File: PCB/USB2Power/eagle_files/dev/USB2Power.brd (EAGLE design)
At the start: 12.5 x 20 mm, 7 parts, among them SW1 PCM12SMTR

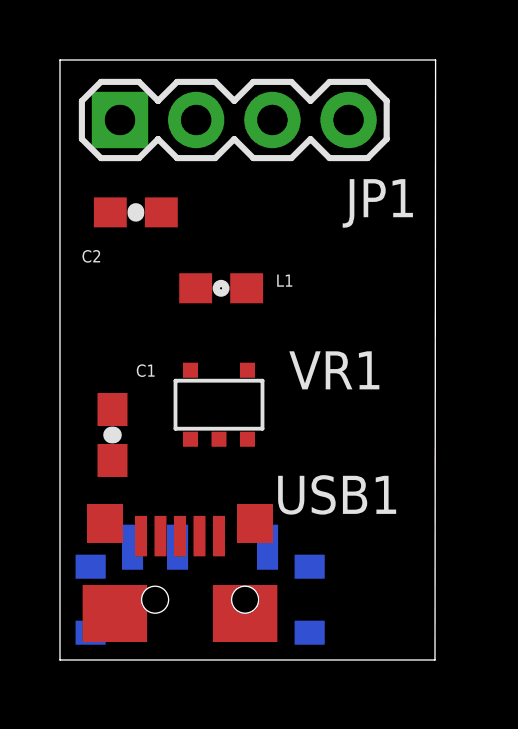
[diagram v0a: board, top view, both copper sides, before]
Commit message: USB2Power board components placed and ready for routing.
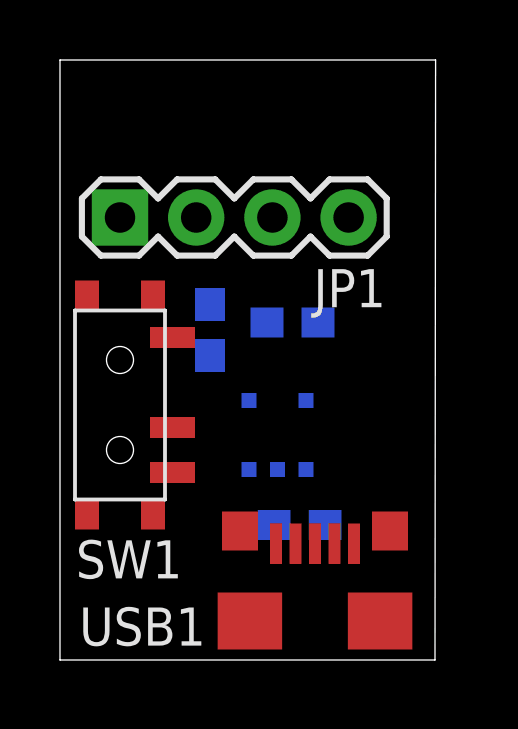
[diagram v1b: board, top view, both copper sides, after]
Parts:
- moved SW1 7.02 mm to (2.00, 8.50), flipped to the top, turned to 270 degrees
- moved C1 6.92 mm to (7.99, 4.50), flipped to the bottom, turned to 180 degrees
- moved C2 4.63 mm to (5.00, 11.0), flipped to the bottom, turned to 270 degrees
- moved USB1 4.51 mm to (8.50, 2.25)
- moved JP1 3.25 mm to (2.00, 14.8)
- moved L1 2.64 mm to (7.75, 11.2), flipped to the bottom
- moved VR1 2.20 mm to (7.25, 7.50), flipped to the bottom
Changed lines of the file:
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@@
 </autorouter>
 <elements>
-<element name="C1" library="SparkFun-Capacitors" package="0603-CAP" value="" x="1.75" y="7.5" smashed="yes" rot="R270">
-<attribute name="NAME" x="2.531" y="9.442" size="0.4064" layer="25" font="vector"/>
-<attribute name="VALUE" x="0.607" y="8.516" size="0.4064" layer="27" font="vector" rot="R270"/>
+<element name="C1" library="SparkFun-Capacitors" package="0603-CAP" value="" x="7.99" y="4.5" smashed="yes" rot="MR180">
+<attribute name="NAME" x="5.711" y="3.318" size="0.4064" layer="26" font="vector" rot="MR180"/>
+<attribute name="VALUE" x="6.974" y="5.643" size="0.4064" layer="28" font="vector" rot="MR180"/>
 </element>
-<element name="C2" library="SparkFun-Capacitors" package="0603-CAP" value="" x="2.53" y="14.92" smashed="yes">
-<attribute name="NAME" x="0.721" y="13.252" size="0.4064" layer="25" font="vector"/>
-<attribute name="VALUE" x="1.514" y="13.777" size="0.4064" layer="27" font="vector"/>
+<element name="C2" library="SparkFun-Capacitors" package="0603-CAP" value="" x="5" y="11" smashed="yes" rot="MR270">
+<attribute name="NAME" x="4.021" y="13.058" size="0.4064" layer="26" font="vector" rot="MR180"/>
+<attribute name="VALUE" x="6.143" y="12.016" size="0.4064" layer="28" font="vector" rot="MR270"/>
 </element>
-<element name="JP1" library="SparkFun-Connectors" package="1X04" value="" x="2" y="18" smashed="yes">
-<attribute name="NAME" x="9.5038" y="14.7588" size="1.27" layer="25" ratio="10"/>
-<attribute name="VALUE" x="0.73" y="14.825" size="1.27" layer="27"/>
+<element name="JP1" library="SparkFun-Connectors" package="1X04" value="" x="2" y="14.75" smashed="yes">
+<attribute name="NAME" x="8.4538" y="11.7588" size="1.27" layer="25" ratio="10"/>
+<attribute name="VALUE" x="0.73" y="11.575" size="1.27" layer="27"/>
 </element>
-<element name="L1" library="SparkFun-Passives" package="0603" value="" x="5.37" y="12.39" smashed="yes">
-<attribute name="PROD_ID" value="RES-07859" x="5.37" y="12.39" size="1.778" layer="27" display="off"/>
-<attribute name="NAME" x="7.191" y="12.442" size="0.4064" layer="25" font="vector"/>
-<attribute name="VALUE" x="4.354" y="11.247" size="0.4064" layer="27" font="vector"/>
+<element name="L1" library="SparkFun-Passives" package="0603" value="" x="7.75" y="11.25" smashed="yes" rot="MR0">
+<attribute name="PROD_ID" value="RES-07859" x="7.75" y="11.25" size="1.778" layer="28" rot="MR0" display="off"/>
+<attribute name="NAME" x="8.809" y="12.452" size="0.4064" layer="26" font="vector" rot="MR0"/>
+<attribute name="VALUE" x="8.766" y="10.107" size="0.4064" layer="28" font="vector" rot="MR0"/>
 </element>
-<element name="SW1" library="freddyLibr" package="PCM12SMTR" value="PCM12SMTR" x="4.67" y="2.01" smashed="yes" rot="MR0">
-<attribute name="NAME" x="6.24" y="5.13" size="1.27" layer="26" rot="MR0"/>
+<element name="SW1" library="freddyLibr" package="PCM12SMTR" value="PCM12SMTR" x="2" y="8.5" smashed="yes" rot="R270">
+<attribute name="NAME" x="0.53" y="2.72" size="1.27" layer="25"/>
 </element>
-<element name="USB1" library="freddyLibr" package="USB-MICROB-SMT" value="USB-MICROB-SMT5-PIN" x="4" y="2.5" smashed="yes">
-<attribute name="NAME" x="11.35" y="6.14" size="1.27" layer="25" rot="R180"/>
+<element name="USB1" library="freddyLibr" package="USB-MICROB-SMT" value="USB-MICROB-SMT5-PIN" x="8.5" y="2.25" smashed="yes">
+<attribute name="NAME" x="0.64" y="0.48" size="1.27" layer="25"/>
 </element>
-<element name="VR1" library="freddyLibr" package="UJ-5_TSOT" value="" x="5.3" y="8.51" smashed="yes">
-<attribute name="NAME" x="7.63" y="9.02" size="1.27" layer="25"/>
+<element name="VR1" library="freddyLibr" package="UJ-5_TSOT" value="" x="7.25" y="7.5" smashed="yes" rot="MR0">
+<attribute name="NAME" x="5.59" y="7.72" size="1.27" layer="26" rot="MR0"/>
 </element>
 </elements>
@@
 <contactref element="VR1" pad="3"/>
 <contactref element="C1" pad="2"/>
-<wire x1="6.25" y1="7.36" x2="2.42" y2="3.76" width="0" layer="19" extent="1-1"/>
-<wire x1="4.35" y1="7.36" x2="6.25" y2="7.36" width="0" layer="19" extent="1-1"/>
-<wire x1="1.75" y1="6.65" x2="4.35" y2="7.36" width="0" layer="19" extent="1-1"/>
+<wire x1="8.2" y1="6.35" x2="6.3" y2="6.35" width="0" layer="19" extent="1-1"/>
+<wire x1="8.84" y1="4.5" x2="8.2" y2="6.35" width="0" layer="19" extent="1-1"/>
+<wire x1="3.75" y1="6.25" x2="6.3" y2="6.35" width="0" layer="19" extent="1-16"/>
 </signal>
 <signal name="N$2">
 <contactref element="VR1" pad="4"/>
 <contactref element="L1" pad="1"/>
-<wire x1="4.52" y1="12.39" x2="4.35" y2="9.66" width="0" layer="19" extent="1-1"/>
+<wire x1="8.2" y1="8.65" x2="8.6" y2="11.25" width="0" layer="19" extent="1-16"/>
 </signal>
 <signal name="GND">
@@
 <contactref element="USB1" pad="9"/>
 <contactref element="JP1" pad="1"/>
-<wire x1="5.3" y1="7.36" x2="5.3" y2="4.13" width="0" layer="19" extent="1-1"/>
-<wire x1="2" y1="18" x2="5.3" y2="7.36" width="0" layer="19" extent="1-1"/>
-<wire x1="1.68" y1="14.92" x2="2" y2="18" width="0" layer="19" extent="1-1"/>
-<wire x1="1.75" y1="8.35" x2="1.68" y2="14.92" width="0" layer="19" extent="1-1"/>
+<wire x1="5" y1="11.85" x2="2" y2="14.75" width="0" layer="19" extent="16-16"/>
+<wire x1="7.14" y1="4.5" x2="5" y2="11.85" width="0" layer="19" extent="1-16"/>
+<wire x1="7.25" y1="6.35" x2="7.14" y2="4.5" width="0" layer="19" extent="1-1"/>
+<wire x1="9.8" y1="3.88" x2="7.25" y2="6.35" width="0" layer="19" extent="1-1"/>
 </signal>
 <signal name="VIN">
 <contactref element="USB1" pad="5"/>
 <contactref element="SW1" pad="2"/>
-<wire x1="3.92" y1="3.76" x2="2.7" y2="4.13" width="0" layer="19" extent="1-1"/>
+<wire x1="7.2" y1="3.88" x2="3.75" y2="7.75" width="0" layer="19" extent="1-16"/>
 </signal>
 <signal name="VOUT">
@@
 <contactref element="SW1" pad="1"/>
 <contactref element="JP1" pad="2"/>
-<wire x1="6.22" y1="12.39" x2="3.38" y2="14.92" width="0" layer="19" extent="1-1"/>
-<wire x1="4.54" y1="18" x2="6.22" y2="12.39" width="0" layer="19" extent="1-1"/>
-<wire x1="6.92" y1="3.76" x2="4.54" y2="18" width="0" layer="19" extent="1-1"/>
-<wire x1="6.25" y1="9.66" x2="6.22" y2="12.39" width="0" layer="19" extent="1-1"/>
+<wire x1="6.3" y1="8.65" x2="6.9" y2="11.25" width="0" layer="19" extent="1-16"/>
+<wire x1="4.54" y1="14.75" x2="6.9" y2="11.25" width="0" layer="19" extent="16-16"/>
+<wire x1="5" y1="10.15" x2="6.3" y2="8.65" width="0" layer="19" extent="1-16"/>
+<wire x1="3.75" y1="10.75" x2="5" y2="10.15" width="0" layer="19" extent="16-16"/>
 </signal>
 </signals>
